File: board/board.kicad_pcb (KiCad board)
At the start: 2 copper layers, 21 x 13 mm, 1 part

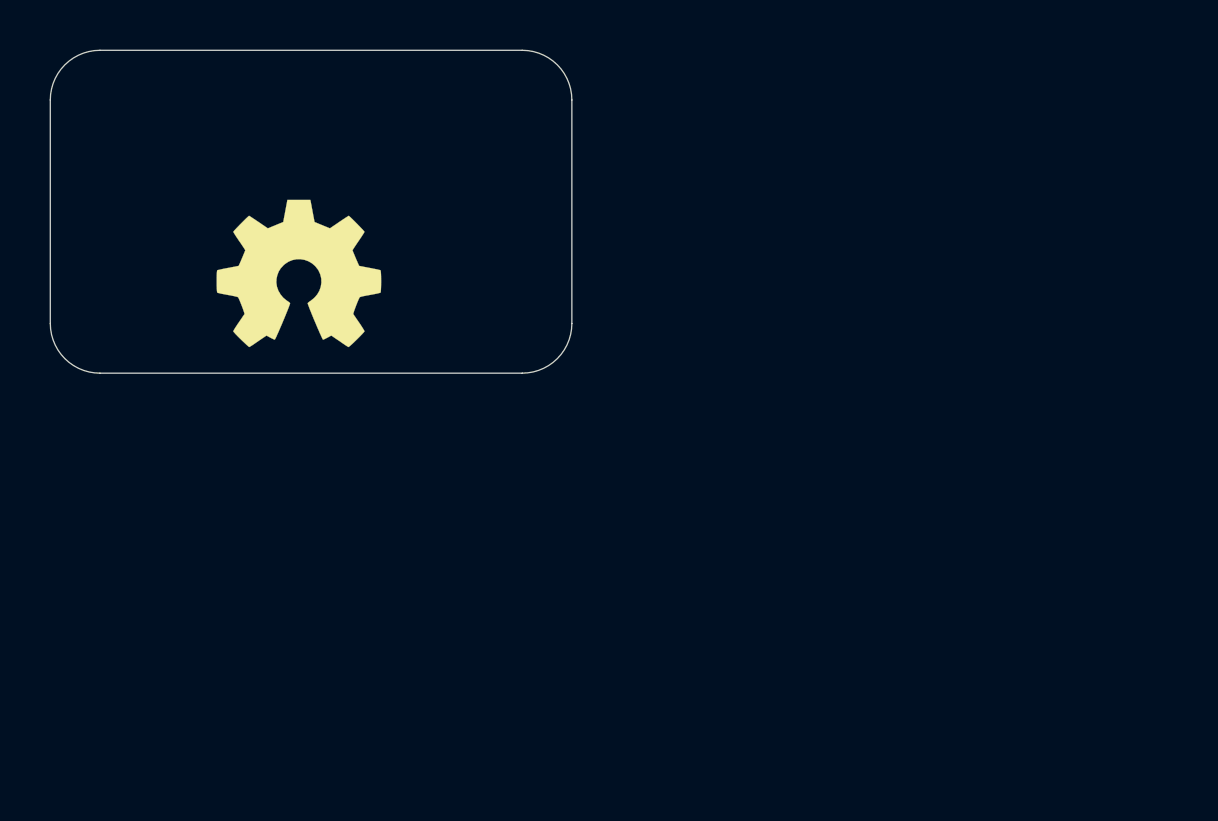
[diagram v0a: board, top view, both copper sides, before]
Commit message: initial
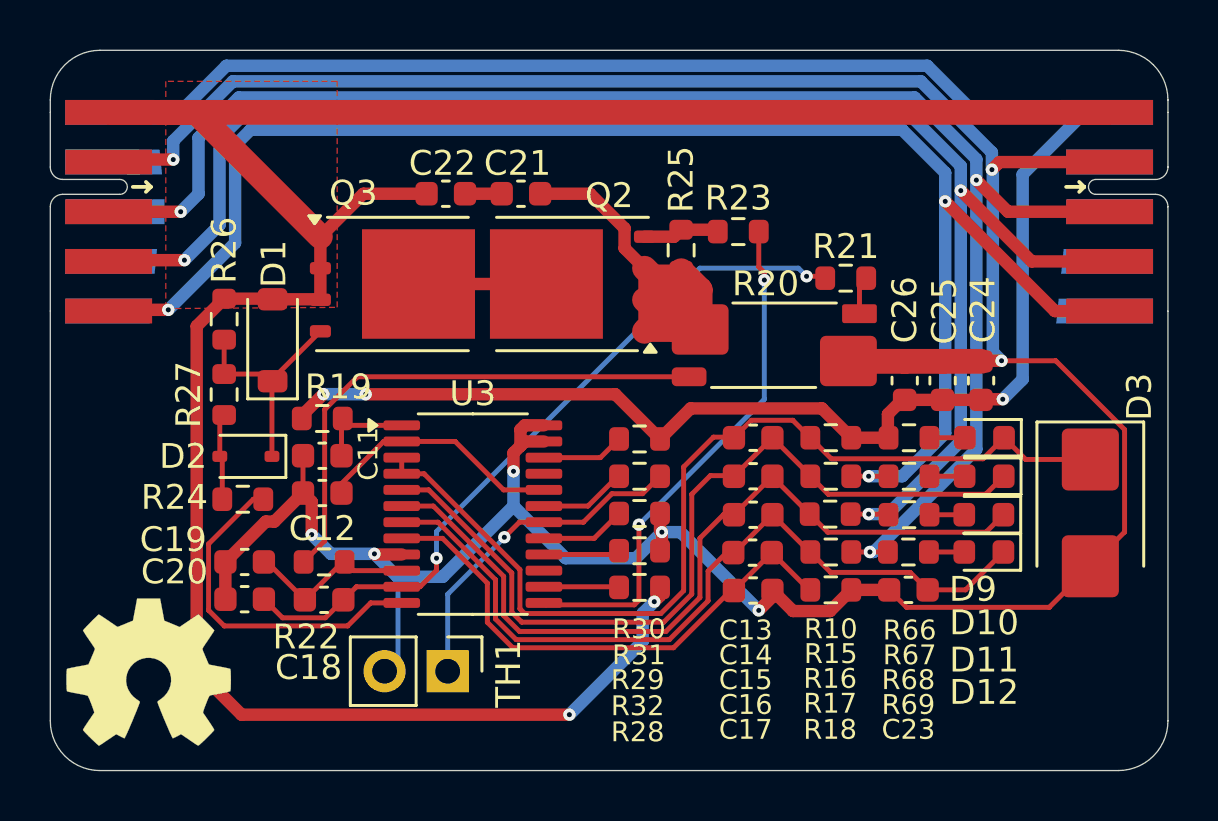
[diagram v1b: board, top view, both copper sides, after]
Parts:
- added C11: 1uF, Capacitor_SMD:C_0603_1608Metric, F.Cu at (150.9, 106.3)
- added C12: 1uF, Capacitor_SMD:C_0603_1608Metric, F.Cu at (150.9, 107.8)
- added C13: 1uF, Capacitor_SMD:C_0603_1608Metric, F.Cu at (168.3, 105.6)
- added C14: 1uF, Capacitor_SMD:C_0603_1608Metric, F.Cu at (168.3, 107.2)
- added C15: 1uF, Capacitor_SMD:C_0603_1608Metric, F.Cu at (168.3, 108.7)
- added C16: 1uF, Capacitor_SMD:C_0603_1608Metric, F.Cu at (168.3, 110.2)
- added C17: 1uF, Capacitor_SMD:C_0603_1608Metric, F.Cu at (168.3, 111.8)
- added C18: 0.1uF, Capacitor_SMD:C_0603_1608Metric, F.Cu at (151.0, 112.1)
- added C19: 0.1uF, Capacitor_SMD:C_0603_1608Metric, F.Cu at (147.8, 110.6)
- added C20: 0.1uF, Capacitor_SMD:C_0603_1608Metric, F.Cu at (147.8, 112.1)
- added C21: 0.1uF, Capacitor_SMD:C_0603_1608Metric, F.Cu at (158.9, 95.8)
- added C22: 0.1uF, Capacitor_SMD:C_0603_1608Metric, F.Cu at (155.9, 95.8)
- added C23: 1uF, Capacitor_SMD:C_0603_1608Metric, F.Cu at (174.6, 111.7)
- added C24: 10uF, Capacitor_SMD:C_0603_1608Metric, F.Cu at (177.5, 103.3)
- added C25: 10uF, Capacitor_SMD:C_0603_1608Metric, F.Cu at (175.9, 103.3)
- added C26: 100nF, Capacitor_SMD:C_0603_1608Metric, F.Cu at (174.4, 103.3)
- added D1: MMSZ5248B, Diode_SMD:D_SOD-123, F.Cu at (148.9, 101.7)
- added D10: C3 LED, LED_SMD:LED_0603_1608Metric, F.Cu at (177.6, 107.2)
- added D11: C2 LED, LED_SMD:LED_0603_1608Metric, F.Cu at (177.6, 108.7)
- added D12: C1 LED, LED_SMD:LED_0603_1608Metric, F.Cu at (177.6, 110.2)
- added D2: BAS316, Diode_SMD:D_SOD-323, F.Cu at (147.9, 106.3)
- added D3: SMBJ26A-13-F, Diode_SMD:D_SMB, F.Cu at (181.9, 108.6)
- added D9: C4 LED, LED_SMD:LED_0603_1608Metric, F.Cu at (177.6, 105.6)
- added J1: 022_battery_cells, on_edge:on_edge_2x05_device, F.Cu at (140.0, 96.5)
- added J2: 022_battery_cells, on_edge:on_edge_2x05_host, F.Cu at (185.0, 96.5)
- added Q2: CSD18534Q5A, Package_TO_SOT_SMD:TDSON-8-1, F.Cu at (161.0, 99.4)
- added Q3: CSD18534Q5A, Package_TO_SOT_SMD:TDSON-8-1, F.Cu at (153.8, 99.4)
- added R10: 33R, Resistor_SMD:R_0603_1608Metric, F.Cu at (171.4, 105.6)
- added R15: 33R, Resistor_SMD:R_0603_1608Metric, F.Cu at (171.4, 107.2)
- added R16: 33R, Resistor_SMD:R_0603_1608Metric, F.Cu at (171.4, 108.7)
- added R17: 33R, Resistor_SMD:R_0603_1608Metric, F.Cu at (171.4, 110.2)
- added R18: 33R, Resistor_SMD:R_0603_1608Metric, F.Cu at (171.4, 111.7)
- added R19: 1k, Resistor_SMD:R_0603_1608Metric, F.Cu at (150.9, 104.8)
- added R20: 15mΩ SHUNT RLP25FEER015, Resistor_SMD:R_Shunt_Vishay_WSK2512_6332Metric_T1.19mm, F.Cu at (169.2, 101.9)
- added R21: 100R, Resistor_SMD:R_0603_1608Metric, F.Cu at (172.0, 99.2)
- added R22: 100R, Resistor_SMD:R_0603_1608Metric, F.Cu at (151.0, 110.6)
- added R23: 5.1k, Resistor_SMD:R_0603_1608Metric, F.Cu at (167.7, 97.3)
- added R24: 5.1k, Resistor_SMD:R_0603_1608Metric, F.Cu at (147.8, 108.1)
- added R25: 10M, Resistor_SMD:R_0603_1608Metric, F.Cu at (165.4, 98.0)
- added R26: 3M, Resistor_SMD:R_0603_1608Metric, F.Cu at (147.0, 100.8)
- added R27: 1M, Resistor_SMD:R_0603_1608Metric, F.Cu at (147.0, 103.9)
- added R28: 470k, Resistor_SMD:R_0603_1608Metric, F.Cu at (163.7, 111.6)
- added R29: 100k, Resistor_SMD:R_0603_1608Metric, F.Cu at (163.7, 108.7)
- added R30: 10k, Resistor_SMD:R_0603_1608Metric, F.Cu at (163.7, 105.7)
- added R31: 10k, Resistor_SMD:R_0603_1608Metric, F.Cu at (163.7, 107.2)
- added R32: 10k, Resistor_SMD:R_0603_1608Metric, F.Cu at (163.7, 110.2)
- added R66: 1k, Resistor_SMD:R_0603_1608Metric, F.Cu at (174.6, 105.6)
- added R67: 1k, Resistor_SMD:R_0603_1608Metric, F.Cu at (174.6, 107.2)
- added R68: 1k, Resistor_SMD:R_0603_1608Metric, F.Cu at (174.6, 108.7)
- added R69: 1k, Resistor_SMD:R_0603_1608Metric, F.Cu at (174.6, 110.2)
- added TH1: 103AT 10k, Connector_PinHeader_2.54mm:PinHeader_1x02_P2.54mm_Vertical, F.Cu at (156.0, 115.0)
- added U3: BQ7791501PWR, Package_SO:TSSOP-24_4.4x7.8mm_P0.65mm, F.Cu at (157.0, 108.7)
- moved LOGO1 17.2 mm to (143.9, 115.0)
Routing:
- net /balancer/C0: track 0.00 -> 134.7 mm, vias 0 -> 8
- net GND: track 0.00 -> 98.0 mm, vias 0 -> 2
- net /balancer/C4: track 0.00 -> 87.3 mm, vias 0 -> 3
- net /balancer/C2: track 0.00 -> 64.4 mm, vias 0 -> 3
- net /balancer/C1: track 0.00 -> 64.2 mm, vias 0 -> 3
- net /balancer/C3: track 0.00 -> 64.0 mm, vias 0 -> 3
- net /balancer/VC4: track 0.00 -> 39.2 mm
- net /balancer/VC3: track 0.00 -> 34.1 mm
- net /balancer/VC2: track 0.00 -> 32.5 mm
- net /balancer/VC1: track 0.00 -> 31.8 mm
- net /balancer/BMS_SRN: track 0.00 -> 29.8 mm, vias 0 -> 2
- net Net-(R20-Pad3): track 0.00 -> 21.7 mm
- net /balancer/VC0: track 0.00 -> 21.4 mm
- net Net-(C21-Pad1): track 0.00 -> 21.1 mm
- net Net-(U3-CHG): track 0.00 -> 21.0 mm, vias 0 -> 2
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- added copper zone on F.Cu, net GND
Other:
- board size 21 x 13 mm -> 45 x 29 mm
